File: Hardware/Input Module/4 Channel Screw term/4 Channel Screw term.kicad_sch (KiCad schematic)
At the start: 22 parts, among them J1 Screw_Terminal_01x06, J2 Screw_Terminal_01x06, J5 Conn_01x12_Male, U1 LTV-847S, U2 74HC7014

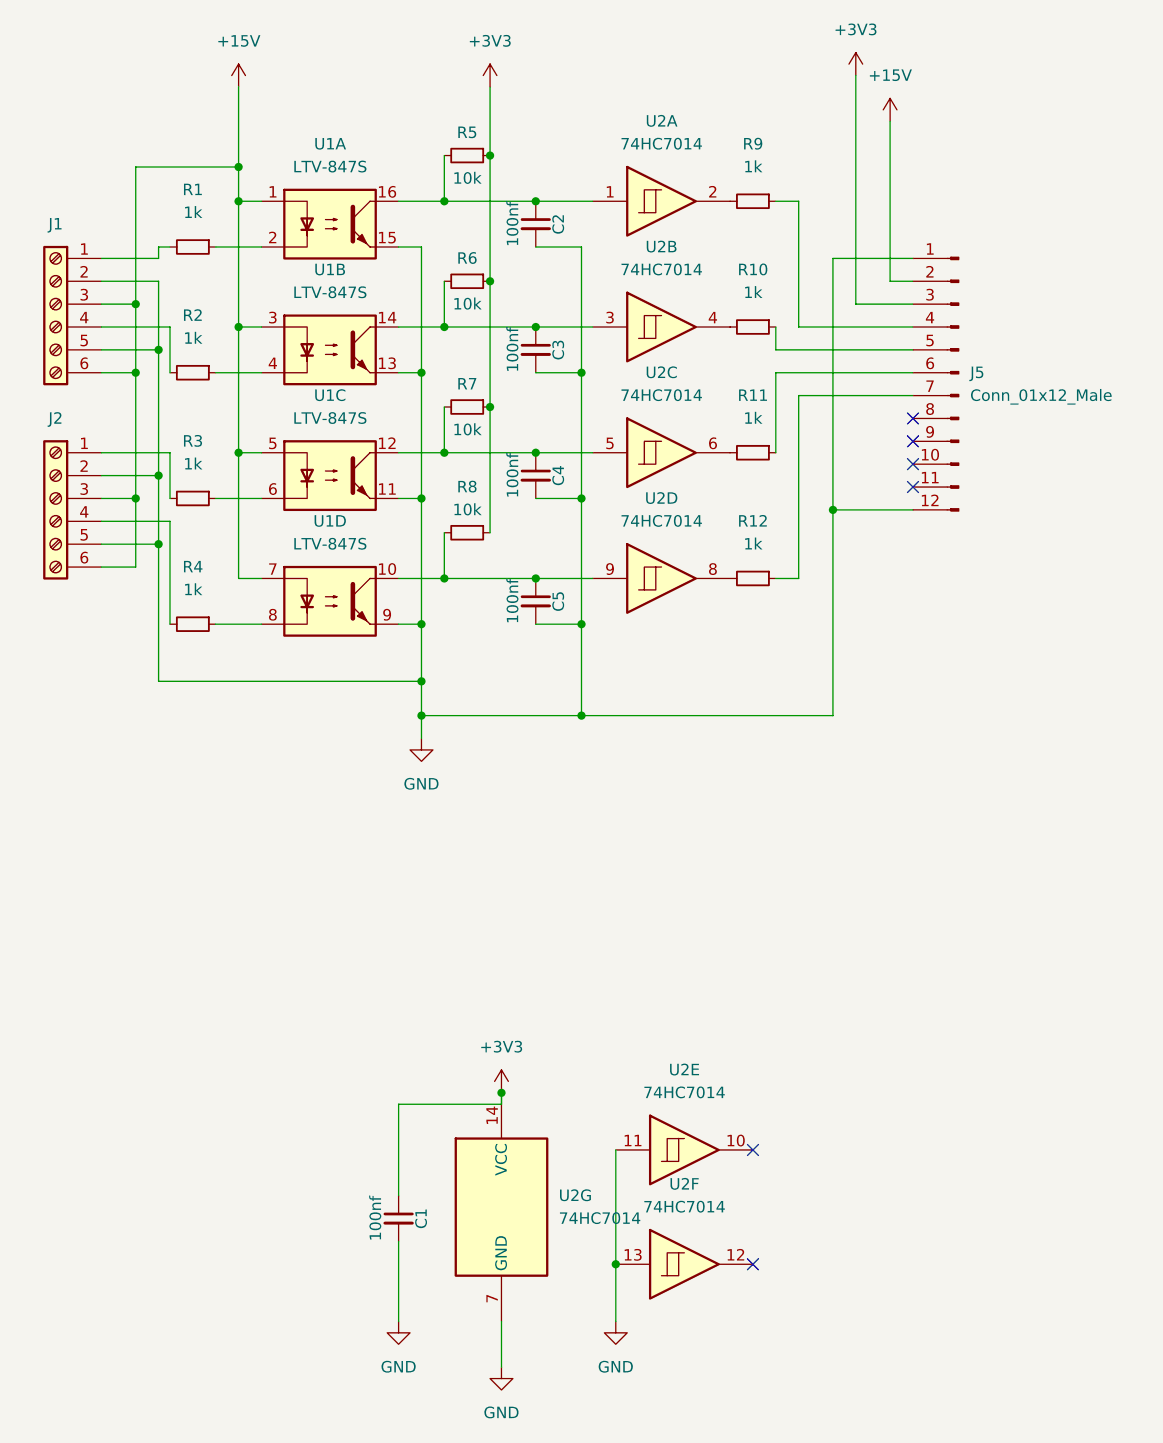
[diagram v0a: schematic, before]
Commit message: Random changes
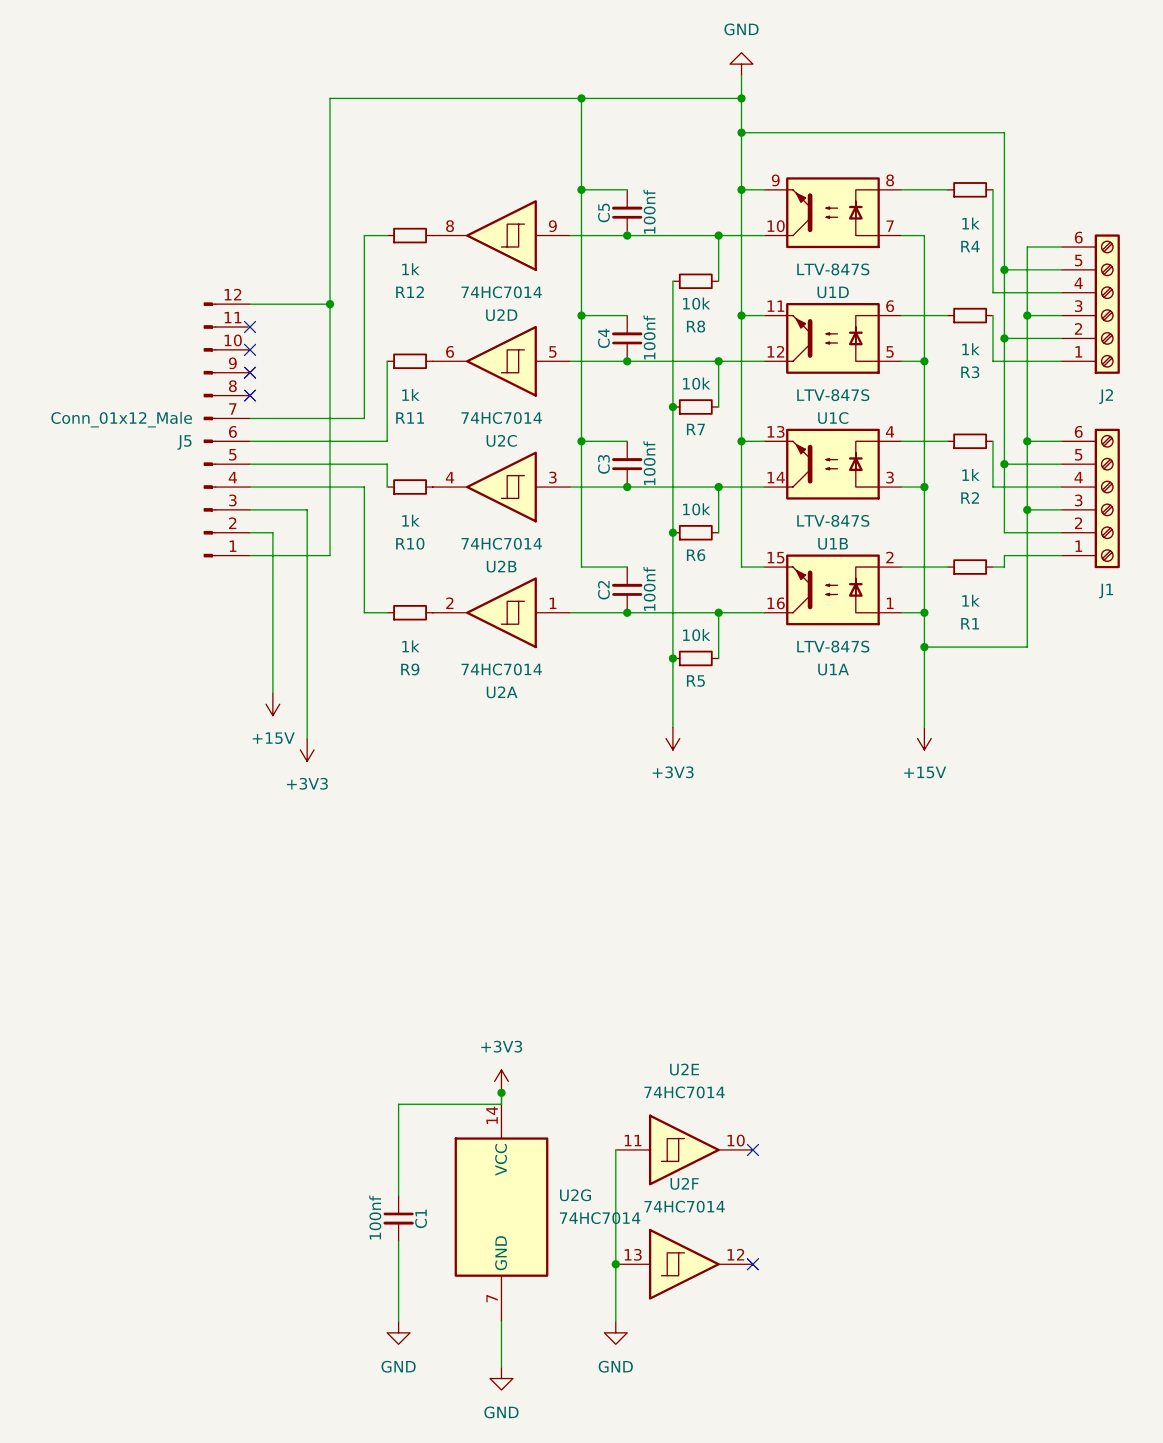
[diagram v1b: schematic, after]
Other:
- moved on the sheet: C2, C3, C4, C5, J1, J2, J5, R1, R10, R11, R12, R2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

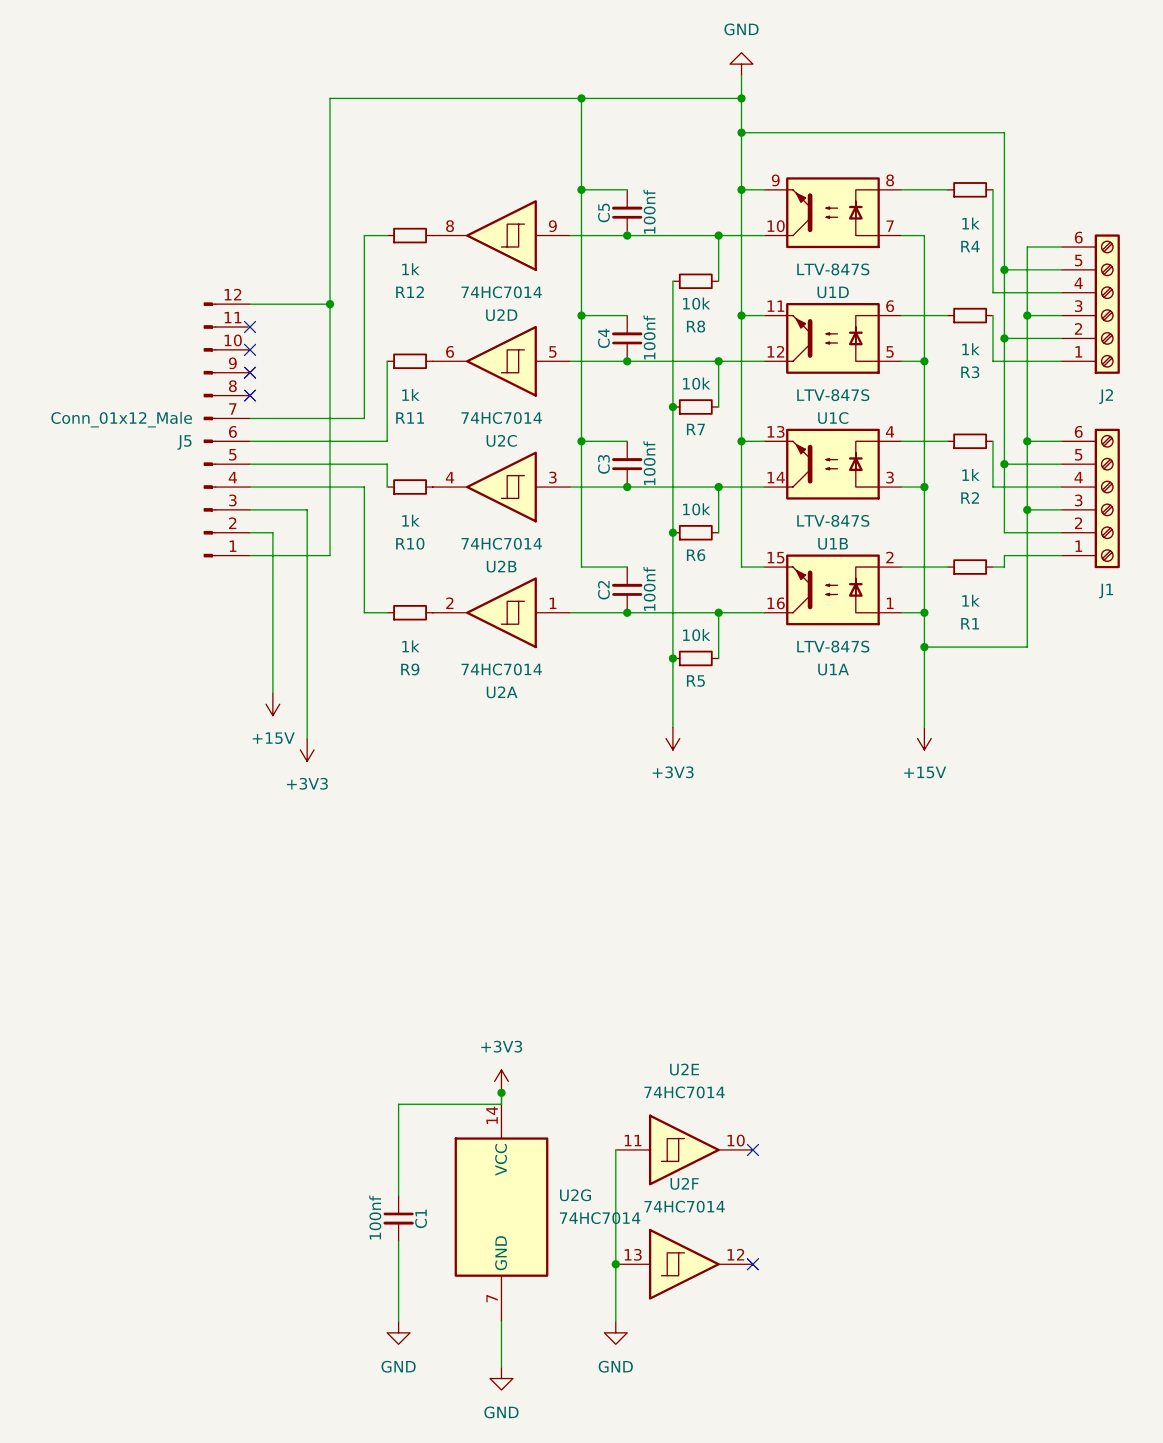
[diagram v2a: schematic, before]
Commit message: v2 work
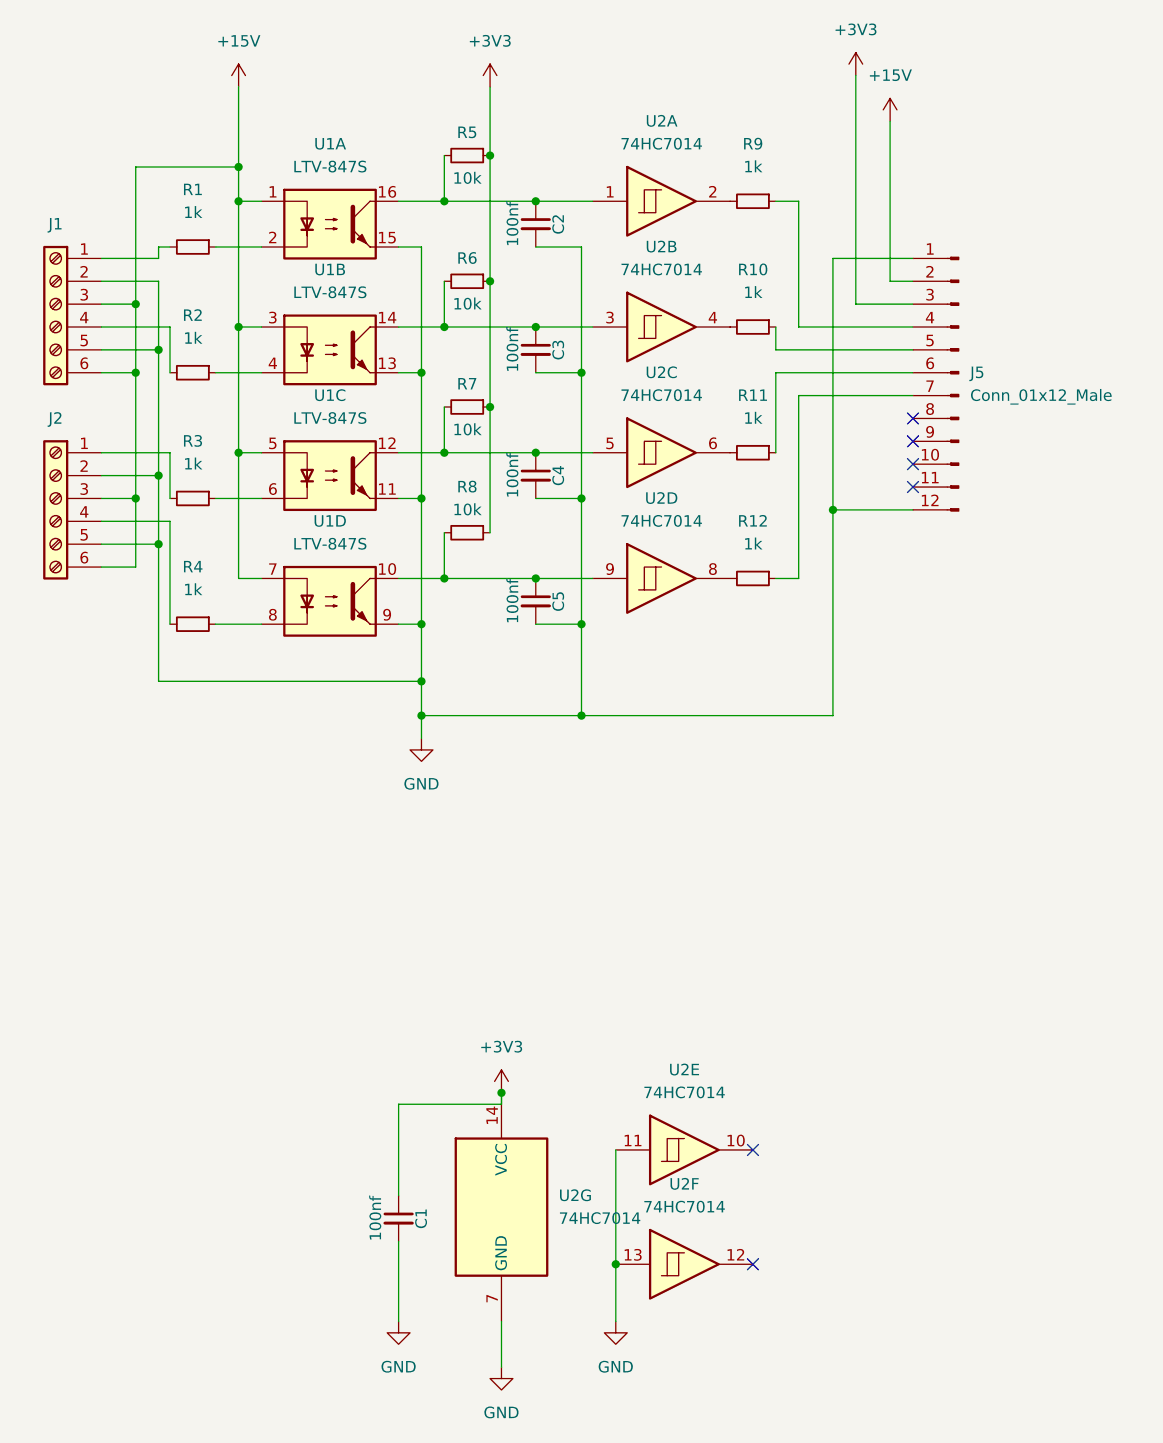
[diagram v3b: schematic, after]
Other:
- moved on the sheet: C2, C3, C4, C5, J1, J2, J5, R1, R10, R11, R12, R2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
